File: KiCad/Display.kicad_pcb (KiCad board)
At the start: 2 copper layers, 44.5 x 67 mm, 31 parts, among them J1 DC, J2 USB-C, M1 OLED1.5-RGB, U1 L86-M33, U2 ESP32-PICO-MINI-02, U3 FT231XQ, U4 LMR16006+FB, U5 QR

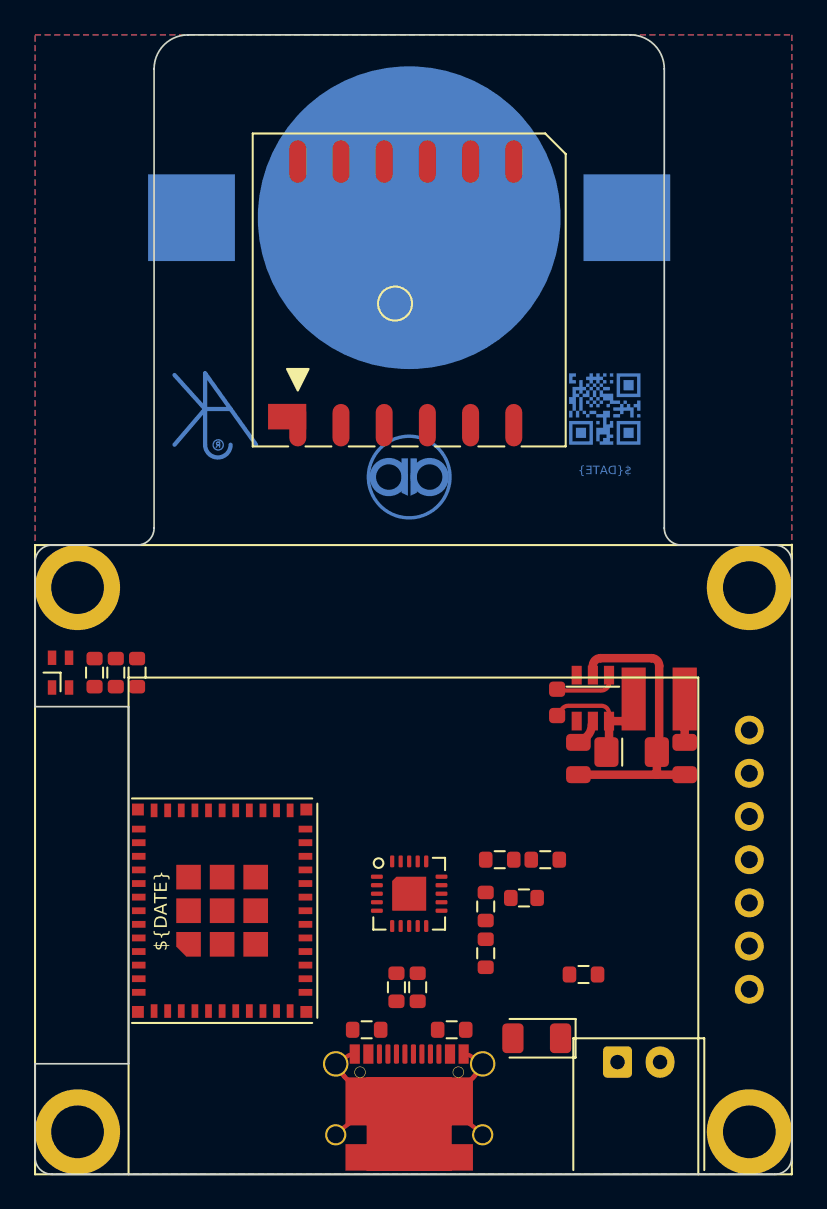
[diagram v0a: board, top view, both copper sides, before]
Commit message: Tracked, needs tidying
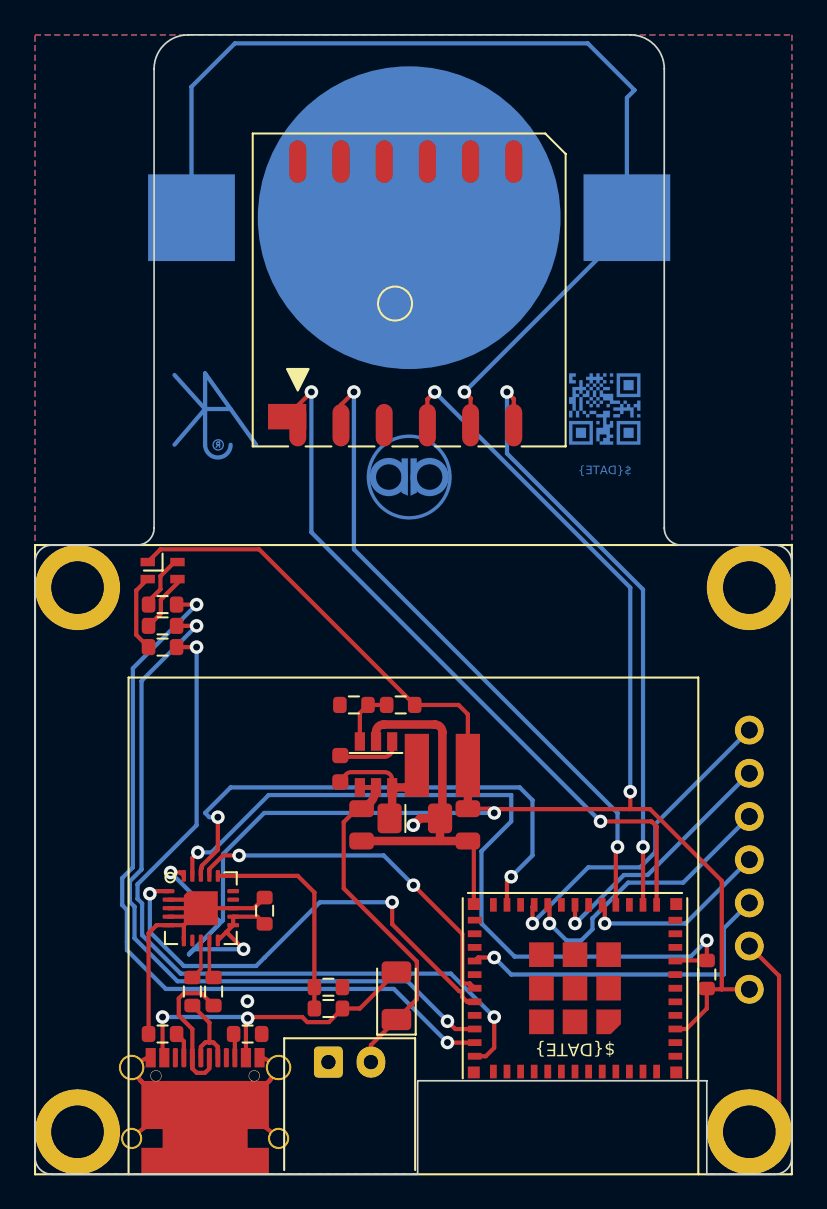
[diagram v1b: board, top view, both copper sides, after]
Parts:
- moved U2 21.2 mm to (109.8, 141.1), turned to 180 degrees
- moved J1 17.0 mm to (96.5, 145.4)
- moved C1 15.3 mm to (91.5, 136.5), turned to 90 degrees
- moved U4 13.3 mm to (98.0, 127.9)
- moved R12 12.5 mm to (96.8, 124.4)
- moved R8 12.5 mm to (99.5, 124.4)
- moved U3 12.3 mm to (87.8, 136.3)
- moved R2 12.0 mm to (85.5, 143.8)
- moved R3 12.0 mm to (90.5, 143.8)
- moved R4 12.0 mm to (88.5, 141.2)
- moved R5 12.0 mm to (87.2, 141.2)
- moved J2 12.0 mm to (88.0, 152.0)
- moved R7 10.4 mm to (95.2, 141.0), turned to 0 degrees
- moved R6 9.80 mm to (95.2, 142.2), turned to 180 degrees
- moved D1 8.62 mm to (99.2, 141.5), turned to 90 degrees
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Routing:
- net +3V3: track 0.00 -> 126.7 mm, vias 0 -> 5
- net Net-(BT1-Pad1): track 0.00 -> 59.9 mm, vias 0 -> 1
- net EN: track 0.00 -> 47.1 mm, vias 0 -> 2
- net R: track 0.00 -> 46.1 mm, vias 0 -> 2
- net B: track 0.00 -> 45.5 mm, vias 0 -> 2
- net G: track 0.00 -> 43.5 mm, vias 0 -> 2
- net GPSRX: track 0.00 -> 42.6 mm, vias 0 -> 2
- net GPSTX: track 0.00 -> 38.9 mm, vias 0 -> 2
- net GND: track 0.00 -> 38.6 mm, vias 0 -> 2
- net TICK: track 0.00 -> 35.6 mm, vias 0 -> 2
- net BOOT: track 0.00 -> 31.7 mm, vias 0 -> 2
- net O: track 0.00 -> 28.3 mm, vias 0 -> 2
- net I: track 0.00 -> 21.3 mm, vias 0 -> 2
- net OLED-MOSI: track 0.00 -> 20.0 mm, vias 0 -> 1
- net VBUS: track 0.00 -> 19.9 mm, vias 0 -> 2
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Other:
- outline, holes or cut-outs redrawn
